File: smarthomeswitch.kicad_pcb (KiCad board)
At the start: 2 copper layers, 124.2 x 64.5 mm, 136 parts, among them J1 Display, J10 DS18B20, J11 Fluxmeter, J12 Electrovalve, J13 Conn_01x04_Male, J15 USB_B_Micro, J17 Conn_ARM_JTAG_SWD_10, J18 RJ45_LED, J2 Conn_01x03_Male, J3 PIR_SR505, J4 Conn_01x04_Male, J5 DS18B20, J6 DS18B20, J7 Fluxmeter, J8 Electrovalve, J9 DS18B20, K1 IM06, Q1 Q_NPN_BCE, Q2 Q_NPN_BCE, Q3 Q_NPN_BCE, T1 Transformer_1P_2S, U1 DS18B20, U2 ATSAM4S2AA, U3 LM3410, U4 LM358, U5 AP5100, U6 ZLDO1117K33TC, U7 ENC28J60x-SS, U8 MTCH101, Y1 12/16 MHz, Y2 25 MHz

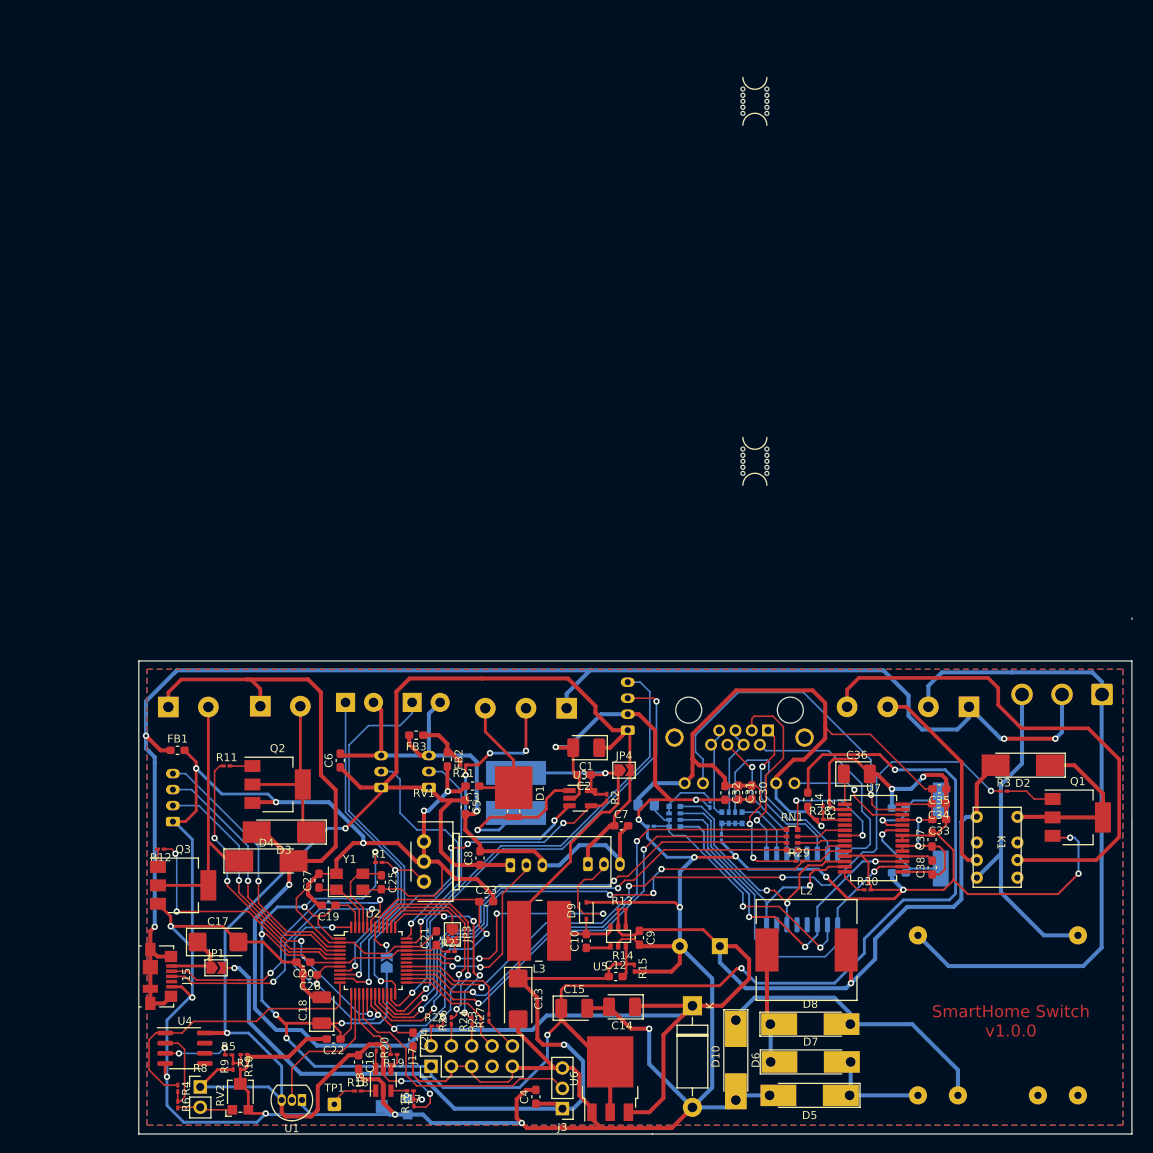
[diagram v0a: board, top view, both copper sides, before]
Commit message: Second version
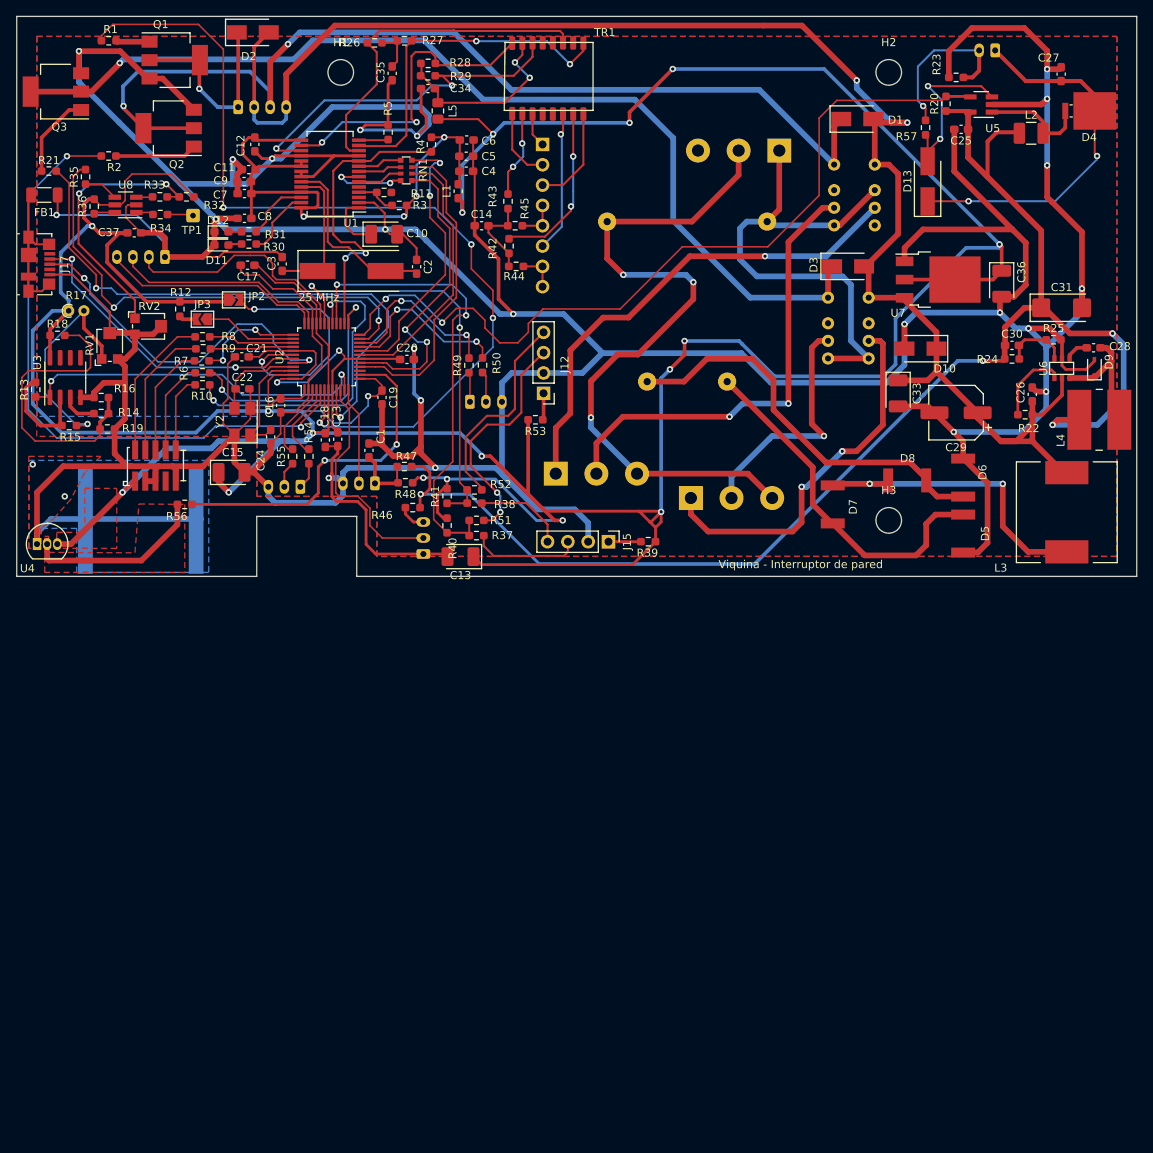
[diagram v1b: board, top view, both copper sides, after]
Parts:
- removed C32, C38: 100n, Capacitor_SMD:C_0603_1608Metric_Pad1.08x0.95mm_HandSolder
- removed C39, C40: 100n, Capacitor_SMD:C_0201_0603Metric_Pad0.64x0.40mm_HandSolder
- removed C41: 1n, Capacitor_SMD:C_0201_0603Metric_Pad0.64x0.40mm_HandSolder
- removed FB2, FB3: FerriteBead, Inductor_SMD:L_0603_1608Metric_Pad1.05x0.95mm_HandSolder
- removed J13: Conn_01x04_Male, Connector_JST:JST_PH_B4B-PH-K_1x04_P2.00mm_Vertical
- removed J18: RJ45_LED, Connector_RJ:RJ45_Amphenol_RJHSE538X
- removed JP1, JP4: SolderJumper_2_Open, Jumper:SolderJumper-2_P1.3mm_Open_TrianglePad1.0x1.5mm
- removed J_AC_INPUT1: Conn_01x03, Connector_JST:JST_NV_B03P-NV_1x03_P5.00mm_Vertical
- removed RN2: R_Pack04, Resistor_SMD:R_Array_Convex_4x0612
- removed RN3: 75, Resistor_SMD:R_Array_Convex_4x0612
- removed RV3: R_Potentiometer, Potentiometer_SMD:Potentiometer_Bourns_TC33X_Vertical
- removed mouse-bite-3mm-slot (x2): VAL**, panelization:mouse-bite-3mm-slot
- added D11: LED, LED_SMD:LED_0603_1608Metric_Pad1.05x0.95mm_HandSolder, F.Cu at (45.6, 68.6)
- added D12: LED, LED_SMD:LED_0603_1608Metric_Pad1.05x0.95mm_HandSolder, F.Cu at (45.6, 66.9)
- added D13: D_Zener, Diode_SMD:D_SMA_Handsoldering, F.Cu at (133.9, 60.6)
- added H1: MountingHole, MountingHole:MountingHole_3.2mm_M3_ISO14580, F.Cu at (60.5, 47.0)
- added H2: MountingHole, MountingHole:MountingHole_3.2mm_M3_ISO14580, F.Cu at (129.0, 47.0)
- added H3: MountingHole, MountingHole:MountingHole_3.2mm_M3_ISO14580, F.Cu at (129.0, 103.0)
- added HS1: Heatsink_Pad, Heatsink:Heatsink_AAVID_573300D00010G_TO-263, B.Cu at (35.5, 102.8)
- added J16: Conn_ARM_JTAG_SWD_10, nqbit:JTAG_50mil, F.Cu at (37.3, 96.1)
- added K2: IM06, footprints:IM06CTS, B.Cu at (124.7, 61.7)
- added R31: R, Resistor_SMD:R_0603_1608Metric_Pad0.98x0.95mm_HandSolder, F.Cu at (49.0, 66.9)
- added R33: 10k, Resistor_SMD:R_0603_1608Metric_Pad0.98x0.95mm_HandSolder, F.Cu at (37.9, 62.6)
- added R34: 4k7, Resistor_SMD:R_0603_1608Metric_Pad0.98x0.95mm_HandSolder, F.Cu at (37.9, 64.8)
- added R35: 100, Resistor_SMD:R_0603_1608Metric_Pad0.98x0.95mm_HandSolder, F.Cu at (28.6, 60.1)
- added R36: 10k, Resistor_SMD:R_0603_1608Metric_Pad0.98x0.95mm_HandSolder, F.Cu at (29.7, 63.8)
- added R37: 100, Resistor_SMD:R_0603_1608Metric_Pad0.98x0.95mm_HandSolder, F.Cu at (77.5, 104.9)
- added R38: 100, Resistor_SMD:R_0603_1608Metric_Pad0.98x0.95mm_HandSolder, F.Cu at (77.2, 100.8)
- added R39: 0, Resistor_SMD:R_0603_1608Metric_Pad0.98x0.95mm_HandSolder, F.Cu at (98.9, 105.7)
- added R40: 1k, Resistor_SMD:R_0603_1608Metric_Pad0.98x0.95mm_HandSolder, F.Cu at (73.8, 103.6)
- added R41: 1k, Resistor_SMD:R_0603_1608Metric_Pad0.98x0.95mm_HandSolder, F.Cu at (73.8, 99.9)
- added R42: R, Resistor_SMD:R_0603_1608Metric_Pad0.98x0.95mm_HandSolder, F.Cu at (81.5, 68.7)
- added R43: R, Resistor_SMD:R_0603_1608Metric_Pad0.98x0.95mm_HandSolder, F.Cu at (81.4, 63.1)
- added R44: R, Resistor_SMD:R_0603_1608Metric_Pad0.98x0.95mm_HandSolder, F.Cu at (82.4, 71.2)
- added R45: R, Resistor_SMD:R_0603_1608Metric_Pad0.98x0.95mm_HandSolder, F.Cu at (82.3, 66.2)
- added R46: R, Resistor_SMD:R_0603_1608Metric_Pad0.98x0.95mm_HandSolder, F.Cu at (69.5, 101.4)
- added R47: R, Resistor_SMD:R_0603_1608Metric_Pad0.98x0.95mm_HandSolder, F.Cu at (68.5, 96.3)
- added R48: R, Resistor_SMD:R_0603_1608Metric_Pad0.98x0.95mm_HandSolder, F.Cu at (68.6, 98.3)
- added R49: R, Resistor_SMD:R_0603_1608Metric_Pad0.98x0.95mm_HandSolder, F.Cu at (76.5, 83.6)
- added R50: R, Resistor_SMD:R_0603_1608Metric_Pad0.98x0.95mm_HandSolder, F.Cu at (78.2, 83.6)
- added R51: 100, Resistor_SMD:R_0603_1608Metric_Pad0.98x0.95mm_HandSolder, F.Cu at (77.5, 103.0)
- added R52: 100, Resistor_SMD:R_0603_1608Metric_Pad0.98x0.95mm_HandSolder, F.Cu at (77.2, 99.2)
- added R53: 0, Resistor_SMD:R_0603_1608Metric_Pad0.98x0.95mm_HandSolder, F.Cu at (84.8, 90.4)
- added R54: R, Resistor_SMD:R_0603_1608Metric_Pad0.98x0.95mm_HandSolder, F.Cu at (56.5, 95.0)
- added R55: R, Resistor_SMD:R_0603_1608Metric_Pad0.98x0.95mm_HandSolder, F.Cu at (54.5, 95.0)
- added R56: R, Resistor_SMD:R_0603_1608Metric_Pad0.98x0.95mm_HandSolder, F.Cu at (41.0, 101.0)
- added R57: 100, Resistor_SMD:R_0603_1608Metric_Pad0.98x0.95mm_HandSolder, F.Cu at (133.6, 53.9)
- C1, C14: value 10u -> C; footprint Capacitor_Tantalum_SMD:CP_EIA-3528-12_Kemet-T_Pad1.50x2.35mm_HandSolder -> Capacitor_SMD:C_0603_1608Metric_Pad1.08x0.95mm_HandSolder
- C10: value 22n -> 10u; footprint Capacitor_SMD:C_0603_1608Metric_Pad1.08x0.95mm_HandSolder -> Capacitor_Tantalum_SMD:CP_EIA-3528-21_Kemet-B_Pad1.50x2.35mm_HandSolder
- C11: value C_Polarized_US -> 100n; footprint Capacitor_THT:CP_Radial_D10.0mm_P5.00mm -> Capacitor_SMD:C_0603_1608Metric_Pad1.08x0.95mm_HandSolder; moved to F.Cu
- C12: value 100p -> 100n
- C13: value 22u -> 10u; footprint Capacitor_Tantalum_SMD:CP_EIA-6032-15_Kemet-U_Pad2.25x2.35mm_HandSolder -> Capacitor_Tantalum_SMD:CP_EIA-3528-12_Kemet-T_Pad1.50x2.35mm_HandSolder
- C17: value 100u -> 100n; footprint Capacitor_Tantalum_SMD:CP_EIA-6032-15_Kemet-U_Pad2.25x2.35mm_HandSolder -> Capacitor_SMD:C_0603_1608Metric_Pad1.08x0.95mm_HandSolder
- C18: value 10u -> 100n; footprint Capacitor_Tantalum_SMD:CP_EIA-3528-12_Kemet-T_Pad1.50x2.35mm_HandSolder -> Capacitor_SMD:C_0603_1608Metric_Pad1.08x0.95mm_HandSolder
- C2, C3: value C -> 22p
- C22, C23, C24: value 100n -> C
- C26, C4, C5, C6, C7, C8: value C -> 100n
- C28: value 22p -> 22n; moved to F.Cu
- C29: value 22p -> C_Polarized_US; footprint Capacitor_SMD:C_0603_1608Metric_Pad1.08x0.95mm_HandSolder -> Capacitor_SMD:CP_Elec_6.3x5.8; moved to F.Cu
- C30: value 100n -> 100p
- C31: value 100n -> 22u; footprint Capacitor_SMD:C_0603_1608Metric_Pad1.08x0.95mm_HandSolder -> Capacitor_Tantalum_SMD:CP_EIA-6032-15_Kemet-U_Pad2.25x2.35mm_HandSolder
- C33: value 100n -> 10u; footprint Capacitor_SMD:C_0603_1608Metric_Pad1.08x0.95mm_HandSolder -> Capacitor_Tantalum_SMD:CP_EIA-3528-12_Kemet-T_Pad1.50x2.35mm_HandSolder
- C36: footprint Capacitor_Tantalum_SMD:CP_EIA-3528-21_Kemet-B_Pad1.50x2.35mm_HandSolder -> Capacitor_Tantalum_SMD:CP_EIA-3528-12_Kemet-T_Pad1.50x2.35mm_HandSolder
- D1: value D_Schottky -> DIODE; footprint Diode_SMD:D_Powermite2_AK -> Diode_SMD:D_SMA
- D10: footprint Diode_THT:D_DO-15_P12.70mm_Horizontal -> Diode_SMD:D_SMA
- D2, D3: footprint Diode_SMD:D_MELF_Handsoldering -> Diode_SMD:D_SMA
- D4: value DIODE -> D_Schottky; footprint Diode_SMD:D_MELF_Handsoldering -> Diode_SMD:D_Powermite2_AK
- D5, D6, D7, D8: footprint Diode_SMD:D_MELF-RM10_Universal_Handsoldering -> gesfluid:DO-213AB
- FB1: footprint Inductor_SMD:L_0603_1608Metric_Pad1.05x0.95mm_HandSolder -> Inductor_SMD:L_1206_3216Metric_Pad1.22x1.90mm_HandSolder
- J1: value Display -> Conn_Eth; footprint Connector_JST:JST_PH_B4B-PH-K_1x04_P2.00mm_Vertical -> Connector_PinHeader_2.54mm:PinHeader_1x08_P2.54mm_Vertical
- J10: value DS18B20 -> Conn_01x04_Male; footprint Connector_JST:JST_PH_B3B-PH-K_1x03_P2.00mm_Vertical -> Connector_JST:JST_PH_B4B-PH-K_1x04_P2.00mm_Vertical
- J11: value Fluxmeter -> Conn_UART; footprint TerminalBlock_Phoenix:TerminalBlock_Phoenix_PT-1,5-2-3.5-H_1x02_P3.50mm_Horizontal -> Connector_JST:JST_PH_B3B-PH-K_1x03_P2.00mm_Vertical
- J12: value Electrovalve -> Display; footprint TerminalBlock_Phoenix:TerminalBlock_Phoenix_PT-1,5-2-5.0-H_1x02_P5.00mm_Horizontal -> Connector_PinHeader_2.54mm:PinHeader_1x04_P2.54mm_Vertical; moved to F.Cu
- J15: value USB_B_Micro -> Display; footprint Connector_USB:USB_Micro-B_Molex_47346-0001 -> Connector_PinHeader_2.54mm:PinHeader_1x04_P2.54mm_Vertical
- J17: value Conn_ARM_JTAG_SWD_10 -> USB_B_Micro; footprint Connector_PinHeader_2.54mm:PinHeader_2x05_P2.54mm_Vertical -> Connector_USB:USB_Micro-B_Molex_47346-0001
- J2: value Conn_01x03_Male -> AC_IN; footprint TerminalBlock_Phoenix:TerminalBlock_Phoenix_MKDS-1,5-3-5.08_1x03_P5.08mm_Horizontal -> TerminalBlock:TerminalBlock_bornier-3_P5.08mm
- J3: value PIR_SR505 -> AC_OUT_1; footprint Connector_PinHeader_2.54mm:PinHeader_1x03_P2.54mm_Vertical -> TerminalBlock:TerminalBlock_bornier-3_P5.08mm; moved to B.Cu
- J4: value Conn_01x04_Male -> AC_OUT_2; footprint TerminalBlock_Phoenix:TerminalBlock_Phoenix_MKDS-1,5-4-5.08_1x04_P5.08mm_Horizontal -> TerminalBlock:TerminalBlock_bornier-3_P5.08mm
- J5: value DS18B20 -> Conn_Q_RAD
- J6: value DS18B20 -> Conn_Led; footprint Connector_JST:JST_PH_B3B-PH-K_1x03_P2.00mm_Vertical -> Connector_JST:JST_PH_B2B-PH-K_1x02_P2.00mm_Vertical
- J7: value Fluxmeter -> Conn_RAD_Valves; footprint TerminalBlock_Phoenix:TerminalBlock_Phoenix_PT-1,5-2-3.5-H_1x02_P3.50mm_Horizontal -> Connector_JST:JST_PH_B4B-PH-K_1x04_P2.00mm_Vertical
- J8: value Electrovalve -> Conn_PIR; footprint TerminalBlock_Phoenix:TerminalBlock_Phoenix_PT-1,5-2-5.0-H_1x02_P5.00mm_Horizontal -> Connector_JST:JST_PH_B3B-PH-K_1x03_P2.00mm_Vertical
- J9: value DS18B20 -> Conn_RAD_TEMP
- JP2, L5: moved to F.Cu
- K1: moved to B.Cu
- L1: footprint Inductor_SMD:L_Wuerth_WE-PD2-Typ-L -> Inductor_SMD:L_0603_1608Metric_Pad1.05x0.95mm_HandSolder; moved to F.Cu
- L2: value 4.7mH -> L; footprint Inductor_SMD:L_12x12mm_H8mm -> Inductor_SMD:L_1210_3225Metric_Pad1.42x2.65mm_HandSolder
- L3: value 22uH -> 4.7mH; footprint Inductor_SMD:L_Wuerth_WE-PD2-Typ-L -> Inductor_SMD:L_12x12mm_H8mm
- L4: value L -> 22uH; footprint Inductor_SMD:L_0603_1608Metric_Pad1.05x0.95mm_HandSolder -> Inductor_SMD:L_Wuerth_WE-PD2-Typ-L
- R1: value R -> 270; footprint Resistor_SMD:R_0201_0603Metric_Pad0.64x0.40mm_HandSolder -> Resistor_SMD:R_0603_1608Metric_Pad0.98x0.95mm_HandSolder
- R10, R32, R6, R7, R9: value R -> 100; footprint Resistor_SMD:R_0201_0603Metric_Pad0.64x0.40mm_HandSolder -> Resistor_SMD:R_0603_1608Metric_Pad0.98x0.95mm_HandSolder
- R11: value 270 -> 100; footprint Resistor_SMD:R_0201_0603Metric_Pad0.64x0.40mm_HandSolder -> Resistor_SMD:R_0603_1608Metric_Pad0.98x0.95mm_HandSolder
- R12: value 270 -> 10k; footprint Resistor_SMD:R_0201_0603Metric_Pad0.64x0.40mm_HandSolder -> Resistor_SMD:R_0603_1608Metric_Pad0.98x0.95mm_HandSolder
- R13: value 10k -> R; footprint Resistor_SMD:R_0201_0603Metric_Pad0.64x0.40mm_HandSolder -> Resistor_SMD:R_0603_1608Metric_Pad0.98x0.95mm_HandSolder
- R14: value 49.9 -> R; footprint Resistor_SMD:R_0201_0603Metric_Pad0.64x0.40mm_HandSolder -> Resistor_SMD:R_0603_1608Metric_Pad0.98x0.95mm_HandSolder
- R15: value 9.53 -> R; footprint Resistor_SMD:R_0201_0603Metric_Pad0.64x0.40mm_HandSolder -> Resistor_SMD:R_0603_1608Metric_Pad0.98x0.95mm_HandSolder
- R16, R20, R21: footprint Resistor_SMD:R_0201_0603Metric_Pad0.64x0.40mm_HandSolder -> Resistor_SMD:R_0603_1608Metric_Pad0.98x0.95mm_HandSolder
- R17: value 10k -> LDR03; footprint Resistor_SMD:R_0201_0603Metric_Pad0.64x0.40mm_HandSolder -> Resistor_THT:R_Axial_DIN0204_L3.6mm_D1.6mm_P1.90mm_Vertical
- R18: value 4k7 -> R; footprint Resistor_SMD:R_0201_0603Metric_Pad0.64x0.40mm_HandSolder -> Resistor_SMD:R_0603_1608Metric_Pad0.98x0.95mm_HandSolder
- R19: value 100 -> R; footprint Resistor_SMD:R_0201_0603Metric_Pad0.64x0.40mm_HandSolder -> Resistor_SMD:R_0603_1608Metric_Pad0.98x0.95mm_HandSolder
- R2: value 10k -> 270; footprint Resistor_SMD:R_0201_0603Metric_Pad0.64x0.40mm_HandSolder -> Resistor_SMD:R_0603_1608Metric_Pad0.98x0.95mm_HandSolder
- R22, R3, R4: value R -> 10k; footprint Resistor_SMD:R_0201_0603Metric_Pad0.64x0.40mm_HandSolder -> Resistor_SMD:R_0603_1608Metric_Pad0.98x0.95mm_HandSolder
- R23: value R -> 4.02; footprint Resistor_SMD:R_0201_0603Metric_Pad0.64x0.40mm_HandSolder -> Resistor_SMD:R_0603_1608Metric_Pad0.98x0.95mm_HandSolder
- R24: value R -> 49.9; footprint Resistor_SMD:R_0201_0603Metric_Pad0.64x0.40mm_HandSolder -> Resistor_SMD:R_0603_1608Metric_Pad0.98x0.95mm_HandSolder
- R25: value R -> 9.53; footprint Resistor_SMD:R_0201_0603Metric_Pad0.64x0.40mm_HandSolder -> Resistor_SMD:R_0603_1608Metric_Pad0.98x0.95mm_HandSolder
- R26, R27, R28, R29: value R -> 49R9; footprint Resistor_SMD:R_0201_0603Metric_Pad0.64x0.40mm_HandSolder -> Resistor_SMD:R_0603_1608Metric_Pad0.98x0.95mm_HandSolder
- R30: value 2k32 -> R; footprint Resistor_SMD:R_0201_0603Metric_Pad0.64x0.40mm_HandSolder -> Resistor_SMD:R_0603_1608Metric_Pad0.98x0.95mm_HandSolder
- R5: value R -> 2k32; footprint Resistor_SMD:R_0201_0603Metric_Pad0.64x0.40mm_HandSolder -> Resistor_SMD:R_0603_1608Metric_Pad0.98x0.95mm_HandSolder
- R8: value LDR03 -> 100; footprint Connector_PinHeader_2.54mm:PinHeader_1x02_P2.54mm_Vertical -> Resistor_SMD:R_0603_1608Metric_Pad0.98x0.95mm_HandSolder
- RV1: footprint footprints:Potentiometer_Bourns_PTV09A-2_Single_Horizontal -> Potentiometer_SMD:Potentiometer_Bourns_TC33X_Vertical
- T1: value Transformer_1P_2S -> Transformer 12 V 2VA; footprint footprints:12v_transformer -> footprints:12v_transformer_single
- TR1: value WE_LAN_TRANSF_7490100110A -> Transformador LAN Ethernet; footprint footprints:LAN Ethernet Wurth Elektronik -> footprints:SM13072APEL; moved to F.Cu
- U1: value DS18B20 -> ENC28J60x-SS; footprint Package_TO_SOT_THT:TO-92_Inline -> Package_SO:SSOP-28_5.3x10.2mm_P0.65mm
- U3: value LM3410 -> LM358; footprint Package_TO_SOT_SMD:SOT-23-5_HandSoldering -> Package_SO:SOIC-8_3.9x4.9mm_P1.27mm
- U4: value LM358 -> DS18B20; footprint Package_SO:SOIC-8_3.9x4.9mm_P1.27mm -> Package_TO_SOT_THT:TO-92_Inline
- U5: value AP5100 -> LM3410; footprint footprints:SOT26 -> Package_TO_SOT_SMD:SOT-23-5_HandSoldering
- U6: value ZLDO1117K33TC -> AP5100; footprint Package_TO_SOT_SMD:TO-252-3_TabPin2 -> footprints:SOT26
- U7: value ENC28J60x-SS -> ZLDO1117K33TC; footprint Package_SO:SSOP-28_5.3x10.2mm_P0.65mm -> Package_TO_SOT_SMD:TO-252-3_TabPin2
- Y1: value 12/16 MHz -> 25 MHz; footprint Crystal:Crystal_SMD_5032-4Pin_5.0x3.2mm -> Crystal:Crystal_SMD_HC49-SD
- Y2: value 25 MHz -> 12/16 MHz; footprint Crystal:Crystal_SMD_HC49-SD -> Crystal:Crystal_SMD_5032-4Pin_5.0x3.2mm; moved to F.Cu
- moved Q1 147.3 mm to (39.8, 45.5)
- moved D4 139.2 mm to (154.1, 51.8), turned to 180 degrees
- moved R20 137.8 mm to (136.2, 50.9), turned to 90 degrees
- moved C27 137.0 mm to (150.6, 47.2)
- moved D2 132.9 mm to (49.5, 42.0), turned to 0 degrees
- moved R23 132.1 mm to (137.4, 47.6), turned to 180 degrees
- moved C37 125.3 mm to (34.7, 67.1), turned to 0 degrees
- moved R26 122.6 mm to (64.7, 43.3), turned to 0 degrees
- moved R27 122.6 mm to (68.5, 43.1), turned to 0 degrees
- moved R4 122.2 mm to (71.8, 56.0)
- moved J6 119.9 mm to (142.3, 44.2), turned to 180 degrees
- moved C25 118.8 mm to (138.1, 54.1), turned to 180 degrees
- moved R5 117.0 mm to (66.4, 54.5), turned to 90 degrees
- moved C4 116.0 mm to (76.2, 59.3), turned to 0 degrees
- moved C26 115.8 mm to (146.9, 87.2), turned to 90 degrees
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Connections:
- net /ETH_CS renamed /TOP PCB/ETH_CS
- C1 pad 1: VDD -> Net-(C1-Pad1)
- C10 pad 2: Net-(C10-Pad2) -> GND
- C11 pad 1: +12V -> /TOP PCB/ethernet/VDD_ETH
- C12 pad 1: +5V -> /TOP PCB/ethernet/VDD_ETH
- C12 pad 2: Net-(C12-Pad2) -> GND
- C13 pad 1: +5V -> +3V3
- C14 pad 1: +12V -> GND
- C14 pad 2: GND -> Net-(C14-Pad2)
- C16 pad 1: VDD -> +3V3
- C17 pad 1: +5P -> +3V3
- C2 pad 1: +5V -> GND
- C2 pad 2: GND -> Net-(C2-Pad2)
- C20 pad 1: +3V3 -> /TOP PCB/VDD_CORE
- C21 pad 1: +3V3 -> /TOP PCB/VDD_CORE
- C22 pad 1: +3V3 -> Net-(C22-Pad1)
- C23 pad 1: /VDD_CORE -> /TOP PCB/VDD_CORE
- C24 pad 1: /VDD_CORE -> Net-(C24-Pad1)
- C25 pad 1: Net-(C25-Pad1) -> +5V
- C26 pad 1: /VDD_CORE -> +12V
- C27 pad 1: Net-(C27-Pad1) -> /BOTTOM PCB/led_dimmer_out
- C28 pad 1: GND -> Net-(C28-Pad1)
- C29 pad 1: GND -> +12V
- C29 pad 2: Net-(C29-Pad2) -> GND
- C3 pad 1: Net-(C3-Pad1) -> GND
- C3 pad 2: GND -> Net-(C3-Pad2)
- C30 pad 1: /ethernet/VDD_ETH -> +5V
- C30 pad 2: GND -> Net-(C30-Pad2)
- C31 pad 1: /ethernet/VDD_ETH -> +5V
- C33 pad 1: GND -> +12V
- C33 pad 2: /ethernet/VDD_ETH -> GND
- C34 pad 2: /ethernet/VDD_ETH -> Net-(C34-Pad2)
- C35 pad 2: /ethernet/VDD_ETH -> Net-(C35-Pad2)
- C36 pad 1: Net-(C36-Pad1) -> +3V3
- C37 pad 1: /ethernet/VDD_ETH -> +3V3
- C4 pad 1: +5V -> /TOP PCB/ethernet/VDD_ETH
- C5 pad 1: VDD -> /TOP PCB/ethernet/VDD_ETH
- C5 pad 2: GNDD -> GND
- C6 pad 1: VDD -> /TOP PCB/ethernet/VDD_ETH
- C6 pad 2: GNDD -> GND
- C7 pad 1: VDD -> GND
- C7 pad 2: GNDD -> /TOP PCB/ethernet/VDD_ETH
- C8 pad 1: VDD -> GND
- C8 pad 2: GNDD -> /TOP PCB/ethernet/VDD_ETH
- C9 pad 1: +12V -> GND
- C9 pad 2: GND -> /TOP PCB/ethernet/VDD_ETH
- D1 pad 1: Net-(C3-Pad1) -> /BOTTOM PCB/EVALVE_1
- D1 pad 2: Net-(D1-Pad2) -> +12V
- D2 pad 1: Net-(D2-Pad1) -> /BOTTOM PCB/EVALVE_2
- D3 pad 1: Net-(D3-Pad1) -> /BOTTOM PCB/lights
- D4 pad 1: Net-(D4-Pad1) -> /BOTTOM PCB/led_dimmer_out
- D4 pad 2: +12V -> Net-(D4-Pad2)
- D9 pad 1: Net-(C10-Pad2) -> Net-(C28-Pad2)
- FB1 pad 1: GNDPWR -> Net-(FB1-Pad1)
- J1 pad 1: VDD -> Net-(J1-Pad1)
- J1 pad 2: GND -> Net-(J1-Pad2)
- J1 pad 3: /display_sck -> Net-(J1-Pad3)
- J1 pad 4: /display_SDA -> Net-(J1-Pad4)
- J10 pad 1: VDD -> GND
- J10 pad 2: /HOT_TEMP_DATA_2 -> /TOP PCB/pwm_shutter3
- J10 pad 3: GNDD -> /TOP PCB/pwm_shutter2
- J11 pad 1: /Q_RAD2 -> Net-(J11-Pad1)
- J11 pad 2: GNDD -> Net-(J11-Pad2)
- J12 pad 1: +12V -> Net-(J12-Pad1)
- J12 pad 2: Net-(D4-Pad1) -> GND
- J15 pad 1: +5P -> Net-(J15-Pad1)
- J15 pad 2: /DM -> GND
- J15 pad 3: /DP -> Net-(J15-Pad3)
- J15 pad 4: unconnected-(J15-Pad4) -> Net-(J15-Pad4)
- J17 pad 1: +3V3 -> +5P
- J17 pad 2: Net-(J17-Pad2) -> /TOP PCB/DM
- J17 pad 3: GND -> /TOP PCB/DP
- J17 pad 4: Net-(J17-Pad4) -> unconnected-(J17-Pad4)
- J17 pad 6: Net-(J17-Pad6) -> Net-(FB1-Pad1)
- J2 pad 1: GNDPWR -> /BOTTOM PCB/AC_POWER_P
- J2 pad 2: /LED_FB -> /BOTTOM PCB/AC_POWER_N
- J2 pad 3: Net-(C3-Pad1) -> GNDPWR
- J3 pad 1: +5V -> Net-(J3-Pad1)
- J3 pad 2: /pir_switch -> Net-(J3-Pad2)
- J3 pad 3: GND -> /BOTTOM PCB/AC_POWER_N
- J4 pad 1: GNDPWR -> Net-(J4-Pad1)
- J4 pad 2: /AC_POWER_N -> Net-(J4-Pad2)
- J4 pad 3: Net-(J4-Pad3) -> /BOTTOM PCB/AC_POWER_N
- J5 pad 1: VDD -> Net-(J5-Pad1)
- J5 pad 2: /COLD_TEMP_DATA_1 -> Net-(J5-Pad2)
- J5 pad 3: GNDD -> GND
- J6 pad 1: VDD -> /BOTTOM PCB/led_dimmer_out
- J6 pad 2: /HOT_TEMP_DATA_1 -> /BOTTOM PCB/LED_FB
- J7 pad 1: /Q_RAD1 -> /BOTTOM PCB/EVALVE_2
- J7 pad 2: GNDD -> +12V
- J8 pad 1: +12V -> GND
- J8 pad 2: Net-(D3-Pad1) -> /BOTTOM PCB/pir_switch
- J9 pad 1: VDD -> Net-(C1-Pad1)
- J9 pad 2: /COLD_TEMP_DATA_2 -> /BOTTOM PCB/RADIATOR_TEMP
- J9 pad 3: GNDD -> GND
- K1 pad 3: Net-(J4-Pad3) -> Net-(J3-Pad1)
- K1 pad 4: /AC_POWER_P -> /BOTTOM PCB/AC_POWER_P
- K1 pad 5: Net-(K1-Pad5) -> /BOTTOM PCB/AC_POWER_P
- K1 pad 6: Net-(J4-Pad4) -> Net-(J3-Pad2)
- K1 pad 8: Net-(D2-Pad1) -> /BOTTOM PCB/lights
- L1 pad 1: +5V -> +3V3
- L1 pad 2: Net-(D1-Pad2) -> /TOP PCB/ethernet/VDD_ETH
- L2 pad 1: Net-(D7-Pad1) -> +5V
- L2 pad 2: +12V -> Net-(D4-Pad2)
- L3 pad 1: Net-(C10-Pad2) -> Net-(D7-Pad1)
- L3 pad 2: +5V -> +12V
- L4 pad 1: +3V3 -> Net-(C28-Pad2)
- L4 pad 2: /ethernet/VDD_ETH -> +5V
- L5 pad 1: /ethernet/VDD_ETH -> Net-(C34-Pad2)
- L5 pad 2: Net-(C40-Pad2) -> +3V3
- Q1 pad 2: Net-(D2-Pad1) -> /BOTTOM PCB/EVALVE_2
- Q2 pad 2: Net-(D3-Pad1) -> /BOTTOM PCB/EVALVE_1
- Q3 pad 2: Net-(D4-Pad1) -> /BOTTOM PCB/lights
- R1 pad 1: +3V3 -> /TOP PCB/VALVE_OUT_2
- R1 pad 2: /selector_an_input -> Net-(Q1-Pad1)
- R10 pad 1: Net-(R10-Pad1) -> Net-(J16-Pad10)
- R10 pad 2: GND -> /TOP PCB/~{MCLR}
- R11 pad 1: /EVALVE_1 -> unconnected-(R11-Pad1)
- R11 pad 2: Net-(Q2-Pad1) -> /TOP PCB/ethernet/ETH_INT
- R12 pad 1: /EVALVE_2 -> +3V3
- R12 pad 2: Net-(Q3-Pad1) -> Net-(JP3-Pad2)
- R13 pad 1: +12V -> /TOP PCB/LDR_an_input
- R14 pad 1: +5V -> Net-(R14-Pad1)
- R14 pad 2: Net-(C12-Pad2) -> Net-(R14-Pad2)
- R15 pad 1: Net-(C12-Pad2) -> Net-(R13-Pad2)
- R15 pad 2: GND -> Net-(R15-Pad2)
- R16 pad 1: VDD -> GND
- R16 pad 2: Net-(R16-Pad2) -> Net-(R14-Pad2)
- R17 pad 1: Net-(R16-Pad2) -> +3V3
- R17 pad 2: Net-(R17-Pad2) -> Net-(R15-Pad2)
- R18 pad 1: Net-(R18-Pad1) -> +3V3
- R18 pad 2: Net-(R18-Pad2) -> Net-(R14-Pad2)
- R19 pad 1: Net-(R19-Pad1) -> Net-(R14-Pad2)
- R19 pad 2: /touchswitch -> GND
- R2 pad 1: +5V -> /TOP PCB/VALVE_OUT_1
- R2 pad 2: /dimmer -> Net-(Q2-Pad1)
- R20 pad 1: VDD -> +5V
- R20 pad 2: Net-(R20-Pad2) -> /BOTTOM PCB/dimmer
- R21 pad 1: /LED_FB -> /TOP PCB/lights_do
- R21 pad 2: GNDA -> Net-(Q3-Pad1)
- R22 pad 1: +3V3 -> +12V
- R22 pad 2: Net-(JP3-Pad2) -> Net-(R22-Pad2)
- R23 pad 1: Net-(J17-Pad8) -> /BOTTOM PCB/LED_FB
- R23 pad 2: /TDI -> GND
- R24 pad 1: Net-(J17-Pad6) -> +5V
- R24 pad 2: /TDO -> Net-(C30-Pad2)
- R25 pad 1: Net-(J17-Pad2) -> Net-(C30-Pad2)
- R25 pad 2: /TMS -> GND
- R26 pad 1: Net-(J17-Pad4) -> /TOP PCB/ethernet/ETH_RX-
- R26 pad 2: /TCK -> Net-(C35-Pad2)
- R27 pad 1: Net-(J17-Pad10) -> Net-(C35-Pad2)
- R27 pad 2: /~{MCLR} -> /TOP PCB/ethernet/ETH_RX+
- R28 pad 1: /ethernet/VDD_ETH -> ETH_TX-
- R28 pad 2: /ethernet/ETH_INT -> Net-(C34-Pad2)
- R29 pad 1: /ethernet/VDD_ETH -> Net-(C34-Pad2)
- R29 pad 2: /ETH_RST -> /TOP PCB/ethernet/ETH_TX+
- R3 pad 1: /lights -> /TOP PCB/ethernet/VDD_ETH
- R3 pad 2: Net-(Q1-Pad1) -> /TOP PCB/ethernet/ETH_INT
- R30 pad 1: Net-(R30-Pad1) -> Net-(D11-Pad2)
- R30 pad 2: GND -> /BOTTOM PCB/LEDA
- R32 pad 1: unconnected-(R32-Pad1) -> +3V3
- R32 pad 2: /ethernet/ETH_INT -> Net-(R32-Pad2)
- R4 pad 1: /LDR_an_input -> /TOP PCB/ethernet/VDD_ETH
- R4 pad 2: Net-(R4-Pad2) -> /TOP PCB/ETH_RST
- R5 pad 2: Net-(R10-Pad1) -> GND
- R6 pad 1: Net-(R4-Pad2) -> Net-(J16-Pad8)
- R6 pad 2: Net-(R6-Pad2) -> /TOP PCB/TDI
- R7 pad 1: GND -> Net-(J16-Pad6)
- R7 pad 2: Net-(R10-Pad1) -> /TOP PCB/TDO
- R8 pad 1: VDD -> Net-(J16-Pad2)
- R8 pad 2: Net-(R6-Pad2) -> /TOP PCB/TMS
- R9 pad 1: VDD -> Net-(J16-Pad4)
- R9 pad 2: Net-(R10-Pad1) -> /TOP PCB/TCK
- RN1 pad 1: /MOSI -> /TOP PCB/MOSI
- RN1 pad 2: /MISO -> /TOP PCB/MISO
- RN1 pad 3: /SCK -> /TOP PCB/SCK
- RV1 pad 1: /selector_an_input -> Net-(R15-Pad2)
- RV2 pad 1: Net-(R6-Pad2) -> Net-(R32-Pad2)
- T1 pad 1: /AC_POWER_P -> /BOTTOM PCB/AC_POWER_P
- T1 pad 10: unconnected-(T1-Pad10) -> Net-(D5-Pad1)
- T1 pad 5: /AC_POWER_N -> /BOTTOM PCB/AC_POWER_N
- T1 pad 6: Net-(D5-Pad1) -> Net-(D6-Pad1)
- TP1 pad 1: Net-(R18-Pad1) -> Net-(R34-Pad1)
- TR1 pad 1: Net-(J18-Pad3) -> Net-(J1-Pad2)
- TR1 pad 10: Net-(C40-Pad2) -> unconnected-(TR1-Pad10)
- TR1 pad 11: /ethernet/ETH_TX+ -> /TOP PCB/ethernet/ETH_RX-
- TR1 pad 14: /ethernet/ETH_RX- -> /TOP PCB/ethernet/ETH_TX+
- TR1 pad 15: unconnected-(TR1-Pad15) -> Net-(C34-Pad2)
- TR1 pad 16: /ethernet/ETH_RX+ -> ETH_TX-
- TR1 pad 3: Net-(J18-Pad6) -> Net-(J1-Pad1)
- TR1 pad 6: Net-(J18-Pad1) -> Net-(J1-Pad6)
- TR1 pad 8: Net-(J18-Pad2) -> Net-(J1-Pad3)
- TR1 pad 9: /ethernet/ETH_TX- -> /TOP PCB/ethernet/ETH_RX+
- U1 pad 1: GND -> Net-(C10-Pad1)
- U1 pad 2: /Air_temp_data -> GND
- U1 pad 3: VDD -> unconnected-(U1-Pad3)
- U2 pad 10: /Q_RAD1 -> /BOTTOM PCB/pir_switch
- U2 pad 11: /Q_RAD2 -> /TOP PCB/LDR_an_input
- U2 pad 12: /LDR_an_input -> /BOTTOM PCB/RADIATOR_TEMP
- U2 pad 14: /Air_temp_data -> Net-(R56-Pad2)
- U2 pad 15: /touchswitch -> unconnected-(U2-Pad15)
- U2 pad 16: /pir_switch -> /TOP PCB/SCK
- U2 pad 17: /pwm_shutter3 -> /TOP PCB/MOSI
- U2 pad 18: /VDD_CORE -> /TOP PCB/VDD_CORE
- U2 pad 19: /ETH_RST -> /TOP PCB/MISO
- U2 pad 21: /SCK -> /TOP PCB/UTX_D0
- U2 pad 22: /display_sck -> /TOP PCB/URX_D0
- U2 pad 23: /display_SDA -> /TOP PCB/touchswitch
- U2 pad 24: /dimmer -> /BOTTOM PCB/dimmer
- U2 pad 25: /TDI -> /TOP PCB/TDI
- U2 pad 26: /MISO -> /TOP PCB/ETH_RST
- U2 pad 27: /MOSI -> unconnected-(U2-Pad27)
- U2 pad 28: /lights -> /TOP PCB/display_sck
- U2 pad 29: /~{MCLR} -> /TOP PCB/~{MCLR}
- U2 pad 3: /pwm_shutter1 -> /BOTTOM PCB/Q_RADIATOR1
- U2 pad 31: /HOT_TEMP_DATA_2 -> /TOP PCB/display_SDA
- U2 pad 32: /COLD_TEMP_DATA_2 -> /TOP PCB/pwm_shutter3
- U2 pad 35: /COLD_TEMP_DATA_1 -> /TOP PCB/pwm_shutter2
- U2 pad 36: /HOT_TEMP_DATA_1 -> /TOP PCB/pwm_shutter1
- U2 pad 37: /TDO -> /TOP PCB/TDO
- U2 pad 39: /TMS -> /TOP PCB/TMS
- U2 pad 4: /pwm_shutter2 -> /BOTTOM PCB/Q_RADIATOR2
- U2 pad 40: /TCK -> /TOP PCB/TCK
- U2 pad 41: /VDD_CORE -> /TOP PCB/VDD_CORE
- U2 pad 43: /DM -> /TOP PCB/DM
- U2 pad 44: /DP -> /TOP PCB/DP
- U2 pad 45: Net-(C25-Pad1) -> Net-(C22-Pad1)
- U2 pad 46: Net-(C27-Pad1) -> Net-(C24-Pad1)
- U2 pad 48: /VDD_CORE -> /TOP PCB/VDD_CORE
- U2 pad 5: /EVALVE_1 -> /TOP PCB/VALVE_OUT_1
- U2 pad 6: /EVALVE_2 -> /TOP PCB/VALVE_OUT_2
- U2 pad 8: /VDD_CORE -> /TOP PCB/VDD_CORE
- U2 pad 9: /selector_an_input -> /TOP PCB/lights_do
- U3 pad 1: Net-(D1-Pad2) -> /TOP PCB/LDR_an_input
- U3 pad 2: GND -> Net-(R13-Pad2)
- U3 pad 3: /LED_FB -> Net-(R14-Pad1)
- U3 pad 4: /dimmer -> GND
- U3 pad 5: +5V -> unconnected-(U3-Pad5)
- U4 pad 1: /LDR_an_input -> GND
- U4 pad 2: Net-(R4-Pad2) -> /TOP PCB/Air_temp_data
- U4 pad 3: Net-(R5-Pad1) -> +3V3
- U5 pad 1: Net-(C10-Pad1) -> Net-(D4-Pad2)
- U5 pad 3: Net-(C12-Pad2) -> Net-(D13-Pad2)
- U5 pad 4: Net-(R13-Pad2) -> /BOTTOM PCB/dimmer
- U5 pad 5: +12V -> +5V
- U6 pad 1: GND -> Net-(C28-Pad1)
- U6 pad 2: +3V3 -> GND
- U6 pad 3: +12V -> Net-(C30-Pad2)
- U7 pad 1: Net-(C36-Pad1) -> GND
- U7 pad 2: GND -> +3V3
- U7 pad 3: unconnected-(U7-Pad3) -> +12V
- U8 pad 1: Net-(R18-Pad2) -> Net-(R34-Pad2)
- U8 pad 3: Net-(R17-Pad2) -> Net-(R33-Pad2)
- U8 pad 4: Net-(R19-Pad1) -> Net-(R35-Pad1)
- U8 pad 5: VDD -> +3V3
- U8 pad 6: Net-(R20-Pad2) -> Net-(R36-Pad2)
- Y1 pad 1: Net-(C27-Pad1) -> Net-(C3-Pad2)
- Y1 pad 2: GND -> Net-(C2-Pad2)
- Y2 pad 1: Net-(C29-Pad2) -> Net-(C24-Pad1)
- Y2 pad 2: Net-(C28-Pad2) -> GND
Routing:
- net +3V3: track 265.6 -> 550.2 mm, vias 9 -> 18
- net VDD: track 208.5 -> 0.00 mm, vias 4 -> 0
- net GND: track 646.9 -> 839.1 mm
- net GNDPWR: track 183.4 -> 0.00 mm, vias 4 -> 0
- net /ethernet/VDD_ETH: track 130.1 -> 0.00 mm, vias 5 -> 0
- net /BOTTOM PCB/lights: track 0.00 -> 125.8 mm, vias 0 -> 1
- net /BOTTOM PCB/EVALVE_1: track 0.00 -> 125.3 mm, vias 0 -> 2
- net /TOP PCB/VALVE_OUT_2: track 0.00 -> 114.7 mm, vias 0 -> 4
- net /BOTTOM PCB/dimmer: track 0.00 -> 102.9 mm, vias 0 -> 2
- net /lights: track 95.1 -> 0.00 mm, vias 4 -> 0
- net /BOTTOM PCB/AC_POWER_N: track 0.00 -> 89.8 mm, vias 0 -> 3
- net /AC_POWER_N: track 84.3 -> 0.00 mm
- net /TOP PCB/VALVE_OUT_1: track 0.00 -> 79.8 mm, vias 0 -> 2
- net /VDD_CORE: track 77.2 -> 0.00 mm, vias 5 -> 0
- net /ETH_RST: track 76.4 -> 0.00 mm, vias 4 -> 0
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- added copper zone on F.Cu, net +3V3
- added copper zone on F.Cu, net /TOP PCB/Air_temp_data
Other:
- board size 124.2 x 64.5 mm -> 140 x 70 mm
- board text added: "Viquina - Interruptor de pared"
- board text removed: "SmartHome Switch v1.0.0"
